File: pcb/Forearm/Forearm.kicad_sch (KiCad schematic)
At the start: 15 parts, among them J1 Conn_01x02, J2 Conn_01x16_Top, J3 Conn_01x16_Bottom, J9 Conn_01x01, U1 ESP32-S3-DEVKITC-1-N8R2, U2 4754

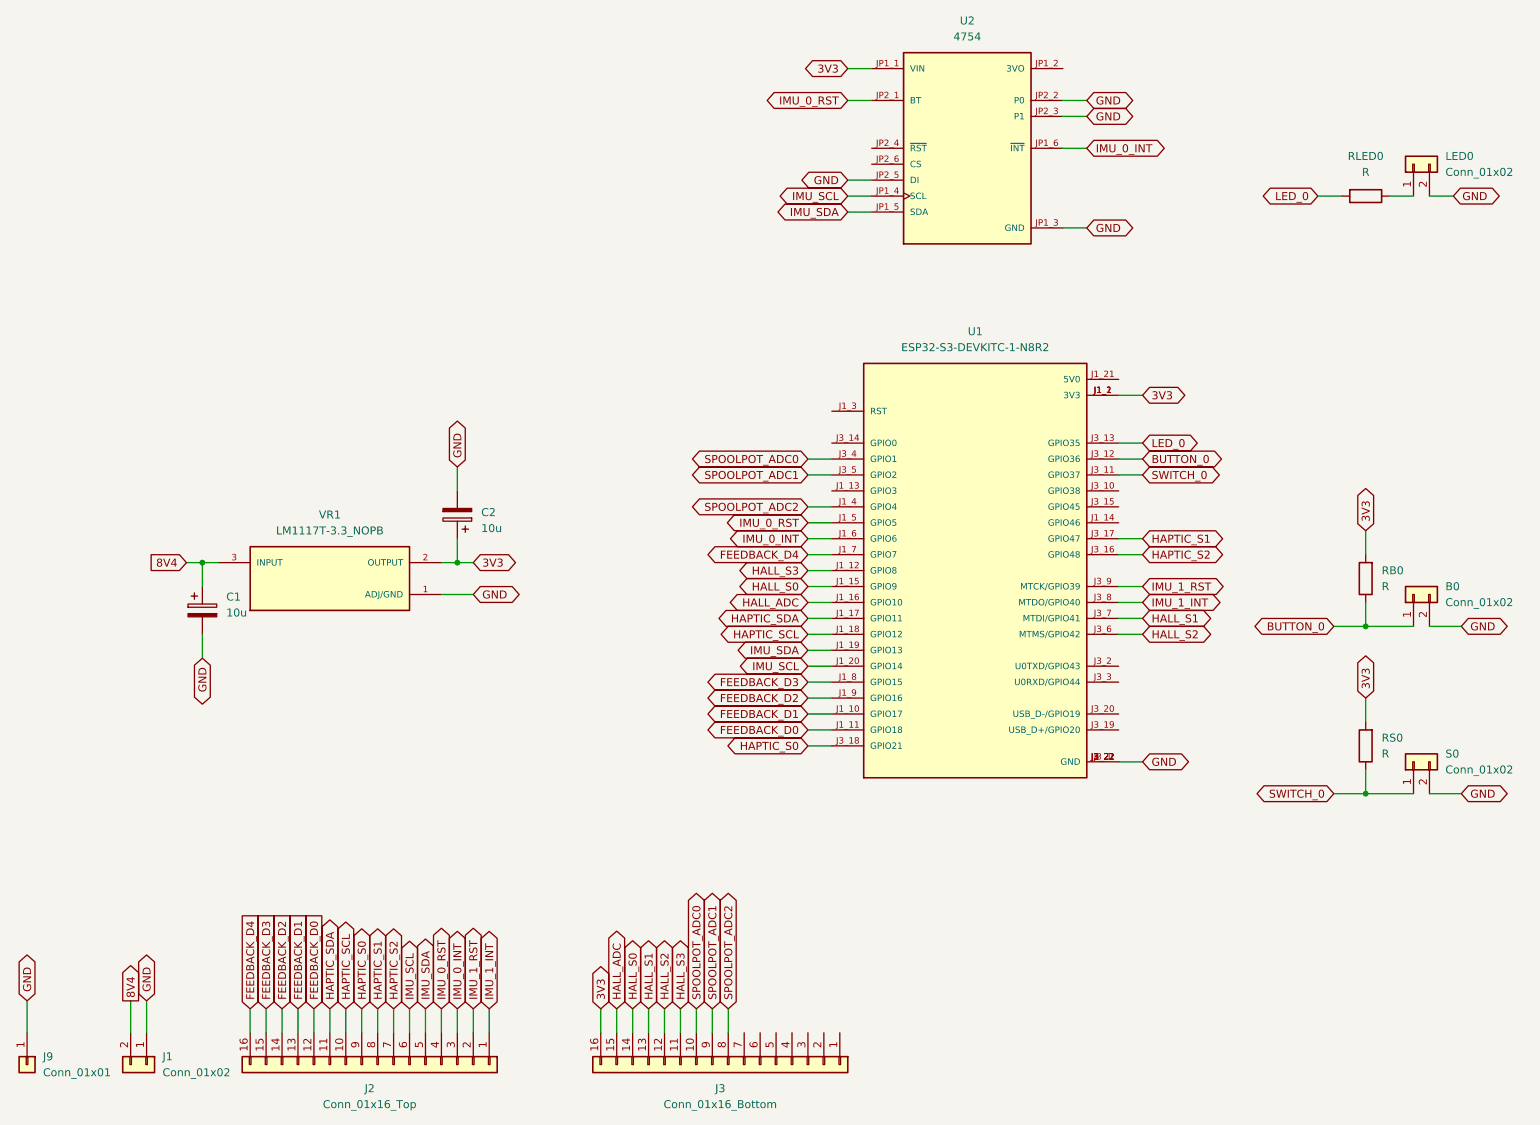
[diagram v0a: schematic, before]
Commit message: revised pcbs in prep for manufacture, rev2
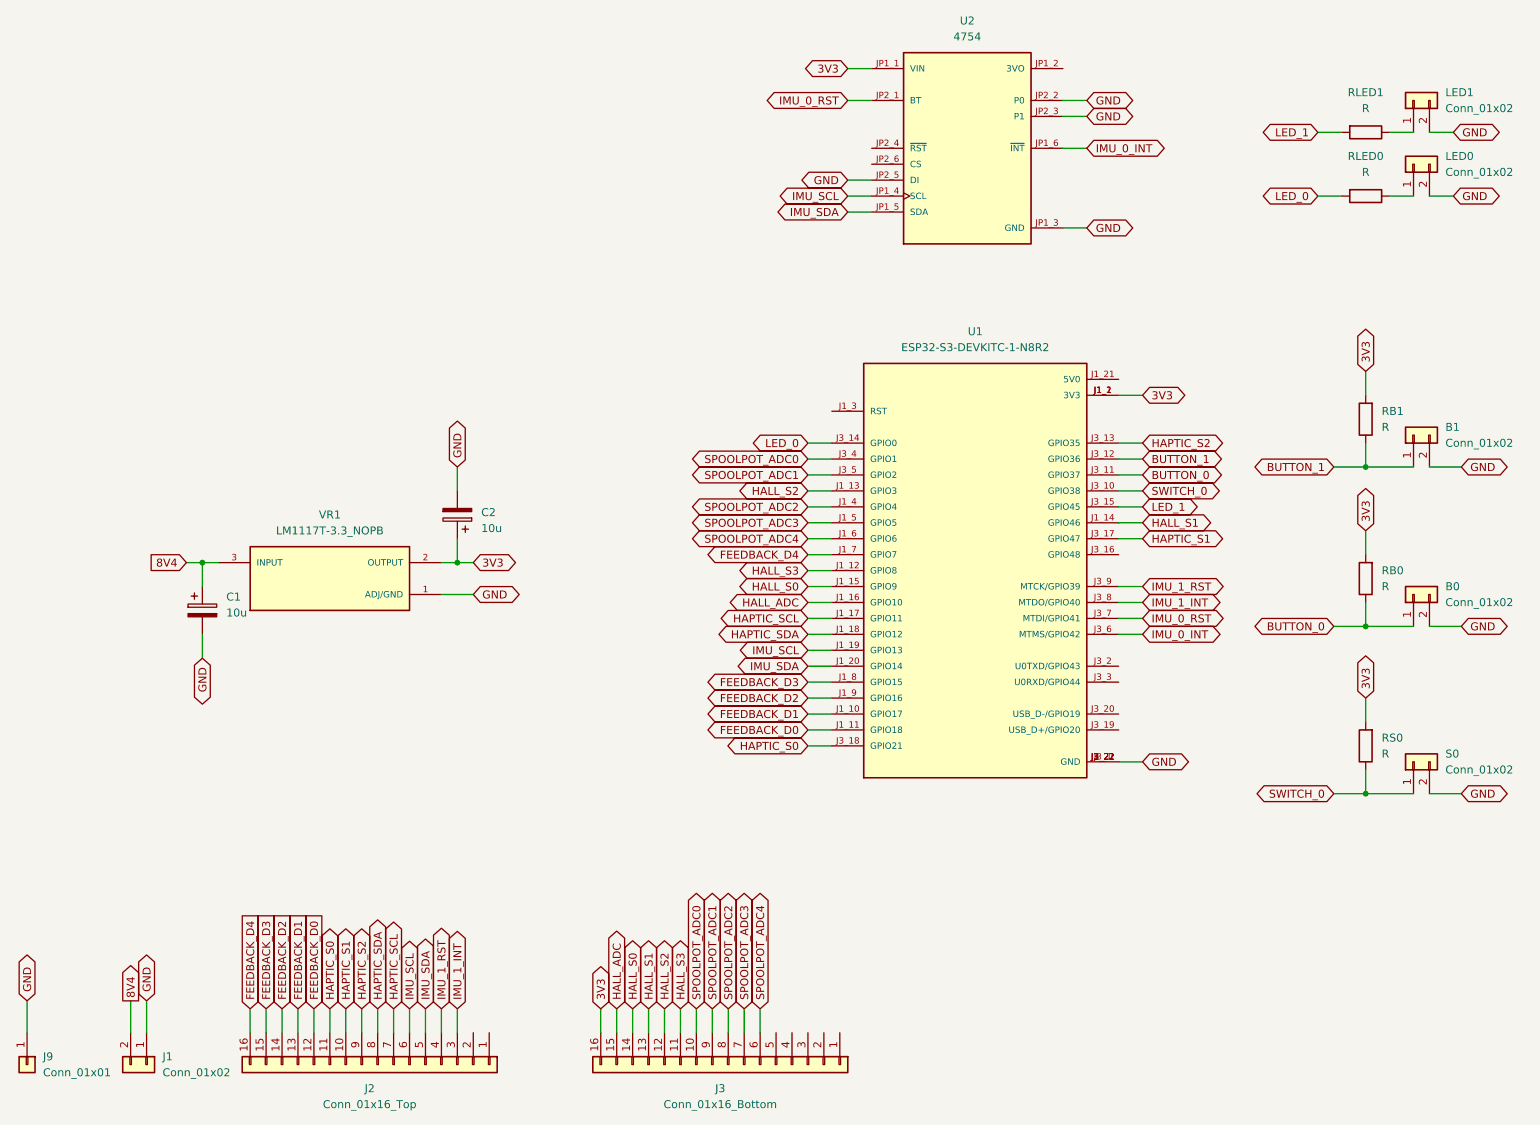
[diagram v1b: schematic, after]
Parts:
- added B1, LED1: Conn_01x02, Connector_PinSocket_2.54mm:PinSocket_1x02_P2.54mm_Vertical, symbol Connector_Generic:Conn_01x02
- added RB1, RLED1: R, Resistor_SMD:R_0402_1005Metric, symbol Device:R
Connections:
- net 3V3: now also RB1.2
- net BUTTON_0: now also U1.J3_11 (GPIO37); no longer U1.J3_12 (GPIO36)
- net GND: now also B1.2 (Pin_2), LED1.2 (Pin_2)
- net HALL_S1: now also U1.J1_14 (GPIO46); no longer U1.J3_7 (MTDI/GPIO41)
- net HALL_S2: now also U1.J1_13 (GPIO3); no longer U1.J3_6 (MTMS/GPIO42)
- net HAPTIC_S0: now also J2.11 (Pin_11); no longer J2.9 (Pin_9)
- net HAPTIC_S1: now also J2.10 (Pin_10); no longer J2.8 (Pin_8)
- net HAPTIC_S2: now also J2.9 (Pin_9), U1.J3_13 (GPIO35); no longer J2.7 (Pin_7), U1.J3_16 (GPIO48)
- net HAPTIC_SCL: now also J2.7 (Pin_7), U1.J1_17 (GPIO11); no longer J2.10 (Pin_10), U1.J1_18 (GPIO12)
- net HAPTIC_SDA: now also J2.8 (Pin_8), U1.J1_18 (GPIO12); no longer J2.11 (Pin_11), U1.J1_17 (GPIO11)
- net IMU_0_INT: now also U1.J3_6 (MTMS/GPIO42); no longer J2.3 (Pin_3), U1.J1_6 (GPIO6)
- net IMU_0_RST: now also U1.J3_7 (MTDI/GPIO41); no longer J2.4 (Pin_4), U1.J1_5 (GPIO5)
- net IMU_1_INT: now also J2.3 (Pin_3); no longer J2.1 (Pin_1)
- net IMU_1_RST: now also J2.4 (Pin_4); no longer J2.2 (Pin_2)
- net IMU_SCL: now also U1.J1_19 (GPIO13); no longer U1.J1_20 (GPIO14)
- net IMU_SDA: now also U1.J1_20 (GPIO14); no longer U1.J1_19 (GPIO13)
- net LED_0: now also U1.J3_14 (GPIO0); no longer U1.J3_13 (GPIO35)
- net SWITCH_0: now also U1.J3_10 (GPIO38); no longer U1.J3_11 (GPIO37)
- net LED_1: now reaches U1.J3_15 (GPIO45)
- net LED_1: now also RLED1.2
- net SPOOLPOT_ADC4: now reaches J3.6 (Pin_6)
- net SPOOLPOT_ADC4: now also U1.J1_6 (GPIO6)
- net SPOOLPOT_ADC3: now reaches J3.7 (Pin_7)
- net SPOOLPOT_ADC3: now also U1.J1_5 (GPIO5)
- new net: LED1.1 (Pin_1), RLED1.1
- new net BUTTON_1: B1.1 (Pin_1), RB1.1, U1.J3_12 (GPIO36)
